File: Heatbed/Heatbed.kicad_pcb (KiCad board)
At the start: 2 copper layers, 35.6 x 30.5 mm, 11 parts, among them J1 Conn_01x04, J2 Conn_01x03, J4 Conn_01x02, Q1 IPP060N06N, Q2 BS170

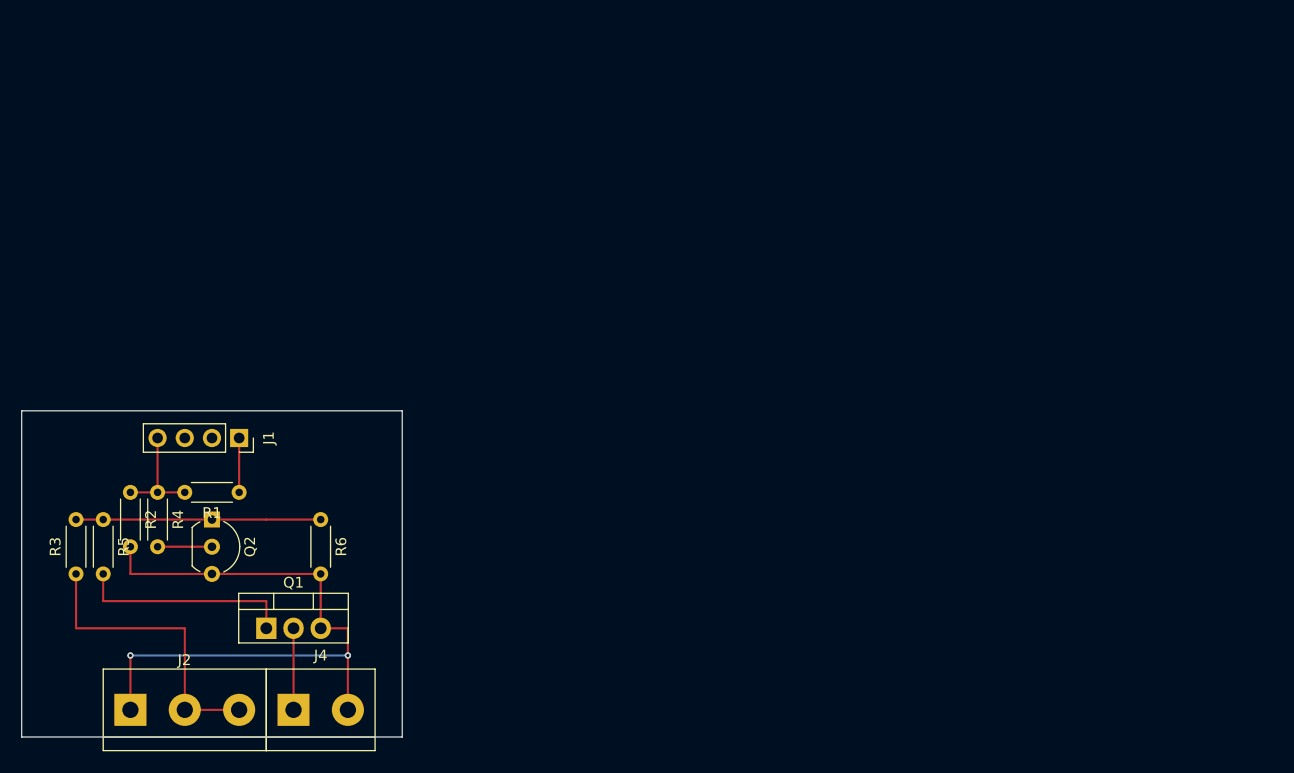
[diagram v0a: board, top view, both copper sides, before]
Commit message: final heatbed circuit
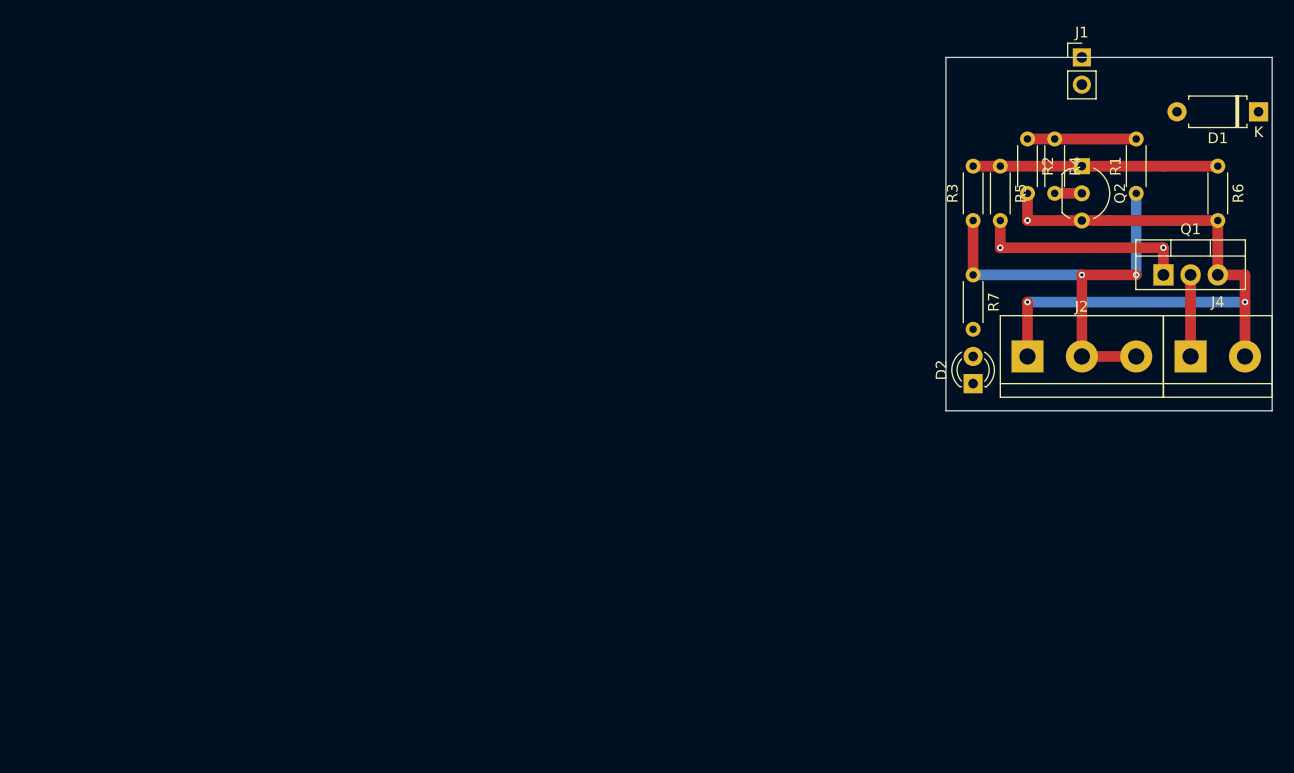
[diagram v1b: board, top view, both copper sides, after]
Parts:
- added D1: D, Diode_THT:D_A-405_P7.62mm_Horizontal, F.Cu at (245.1, 55.9)
- added D2: LED, LED_THT:LED_D3.0mm, F.Cu at (218.4, 81.3)
- added R7: 4k, Resistor_THT:R_Axial_DIN0204_L3.6mm_D1.6mm_P5.08mm_Horizontal, F.Cu at (218.4, 71.1)
- J1: value Conn_01x04 -> Conn_01x02; footprint Connector_PinSocket_2.54mm:PinSocket_1x04_P2.54mm_Vertical -> Connector_PinHeader_2.54mm:PinHeader_1x02_P2.54mm_Vertical
- R2: value 4.7k -> 7.5k
- moved J2 90.1 mm to (223.5, 78.7)
- moved R6 90.1 mm to (241.3, 61.0)
- moved R2 90.1 mm to (223.5, 58.4)
- moved J4 90.1 mm to (238.8, 78.7)
- moved Q1 90.1 mm to (236.2, 71.1)
- moved R3 90.1 mm to (218.4, 66.0)
- moved R4 90.1 mm to (226.1, 58.4)
- moved R5 90.1 mm to (221.0, 61.0)
- moved R1 88.4 mm to (233.7, 63.5), turned to 90 degrees
- moved Q2 87.7 mm to (228.6, 61.0)
- moved J1 86.4 mm to (228.6, 50.8), turned to 0 degrees
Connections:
- J1 pad 1: +15 -> HB_ACTIVE
- R1 pad 1: +15 -> +24
- R1 pad 2: HB_ACTIVE -> Net-(D1-A)
- R2 pad 1: HB_ACTIVE -> Net-(D1-A)
- R4 pad 1: HB_ACTIVE -> Net-(D1-A)
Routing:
- net +24: track 27.9 -> 40.6 mm, vias 0 -> 3
- net HB_ACTIVE: track 10.2 -> 0.00 mm
- net Net-(D1-A): track 0.00 -> 10.2 mm
- net +15: track 5.08 -> 0.00 mm
- net Net-(Q2-G): track 5.08 -> 2.54 mm
- net GND: vias 2 -> 3
- net Net-(Q1-G): vias 0 -> 2
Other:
- board size 35.6 x 30.5 mm -> 30.5 x 33 mm
